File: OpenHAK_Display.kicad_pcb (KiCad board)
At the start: 2 copper layers, 23.4 x 21.7 mm, 13 parts, among them P1 M52-Series_Male_TH_Harwin

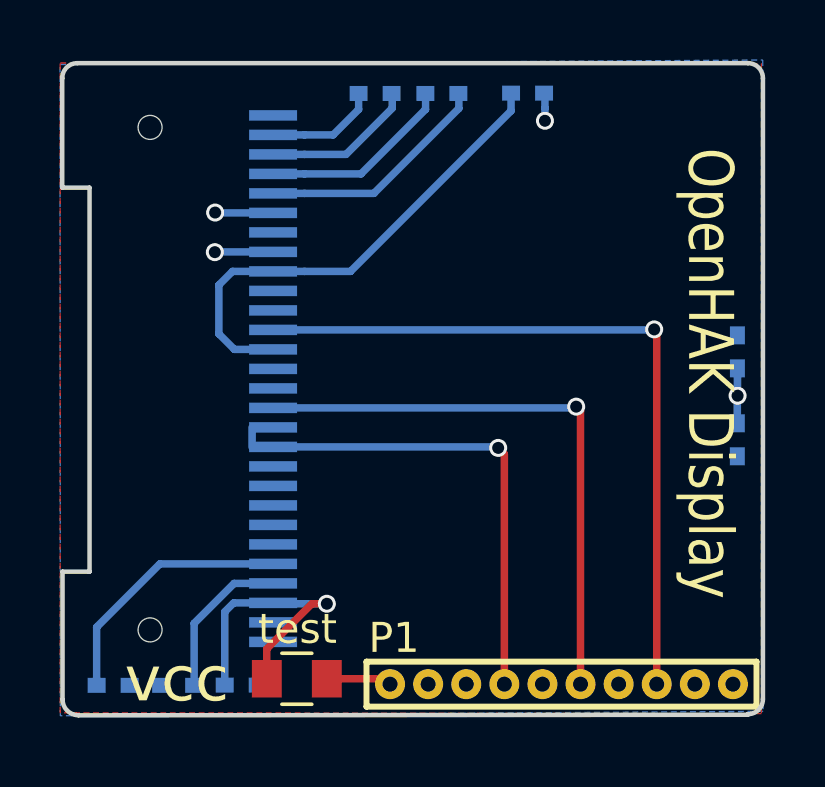
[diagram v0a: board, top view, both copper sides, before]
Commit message: made production files
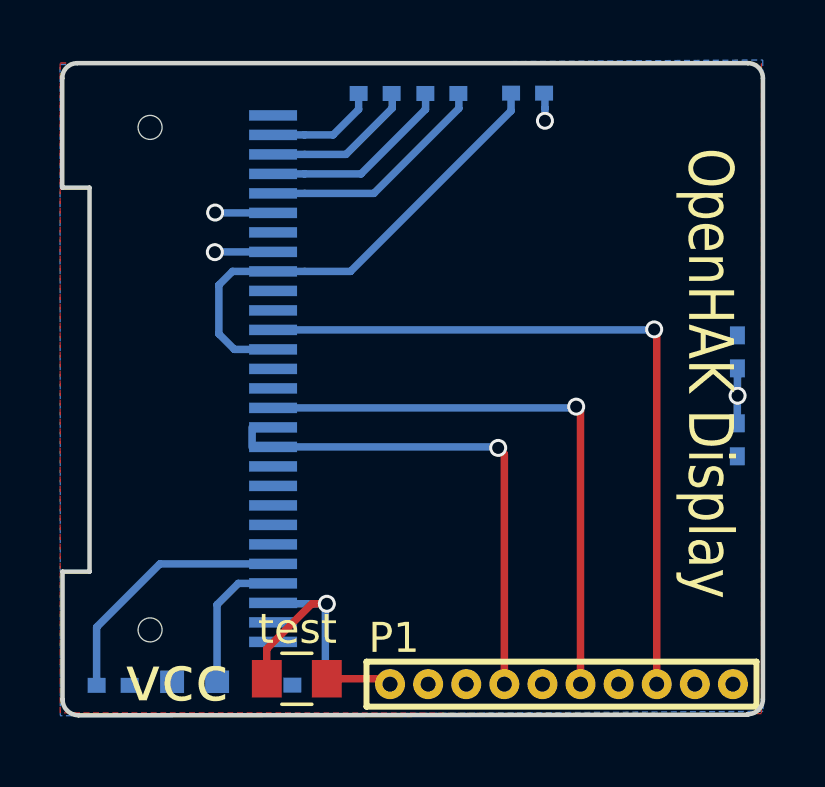
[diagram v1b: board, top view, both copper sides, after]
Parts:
- C3: footprint Capacitors_SMD:C_0402 -> Capacitors_SMD:C_0603
- moved C4 2.25 mm to (125.4, 112.0), turned to 180 degrees
- moved C3 0.58 mm to (121.6, 111.9)
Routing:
- net /VCC: track 9.60 -> 8.16 mm
- net Net-(C3-Pad2): track 5.67 -> 5.15 mm
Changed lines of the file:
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@@
     (thickness 1.6)
     (drawings 30)
-    (tracks 77)
+    (tracks 76)
     (zones 0)
     (modules 13)
@@
     (34 B.Paste user)
     (35 F.Paste user)
-    (36 B.SilkS user)
-    (37 F.SilkS user)
+    (36 B.SilkS user hide)
+    (37 F.SilkS user hide)
     (38 B.Mask user)
     (39 F.Mask user)
@@
     (visible_elements FFFFFF7F)
     (pcbplotparams
-      (layerselection 0x000f4_ffffffff)
+      (layerselection 0x010fc_ffffffff)
       (usegerberextensions false)
       (usegerberattributes false)
@@
   )
   (module Capacitors_SMD:C_0402 (layer B.Cu)
-    (at 121.031338 111.980542)
+    (at 125.405 111.970542 180)
     (descr "Capacitor SMD 0402, reflow soldering, AVX (see smccp.pdf)")
     (tags "capacitor 0402")
     (attr smd)
-    (fp_text reference C3 (at 0.4 -2.05 90) (layer B.SilkS)
-      (effects (font (size 1 1) (thickness 0.15)) (justify mirror))
-    )
-    (fp_text value "4.7uF 16V" (at 0 -1.27) (layer B.Fab)
-      (effects (font (size 1 1) (thickness 0.15)) (justify mirror))
-    )
-    (fp_line (start 1 -0.4) (end -1 -0.4) (layer B.CrtYd) (width 0.05))
-    (fp_line (start 1 -0.4) (end 1 0.4) (layer B.CrtYd) (width 0.05))
-    (fp_line (start -1 0.4) (end -1 -0.4) (layer B.CrtYd) (width 0.05))
-    (fp_line (start -1 0.4) (end 1 0.4) (layer B.CrtYd) (width 0.05))
-    (fp_line (start -0.25 -0.47) (end 0.25 -0.47) (layer B.SilkS) (width 0.12))
-    (fp_line (start 0.25 0.47) (end -0.25 0.47) (layer B.SilkS) (width 0.12))
-    (fp_line (start -0.5 0.25) (end 0.5 0.25) (layer B.Fab) (width 0.1))
-    (fp_line (start 0.5 0.25) (end 0.5 -0.25) (layer B.Fab) (width 0.1))
-    (fp_line (start 0.5 -0.25) (end -0.5 -0.25) (layer B.Fab) (width 0.1))
-    (fp_line (start -0.5 -0.25) (end -0.5 0.25) (layer B.Fab) (width 0.1))
-    (fp_text user %R (at 0 1.27) (layer B.Fab)
-      (effects (font (size 1 1) (thickness 0.15)) (justify mirror))
-    )
-    (pad 2 smd rect (at 0.55 0) (size 0.6 0.5) (layers B.Cu B.Paste B.Mask)
-      (net 5 "Net-(C3-Pad2)"))
-    (pad 1 smd rect (at -0.55 0) (size 0.6 0.5) (layers B.Cu B.Paste B.Mask)
-      (net 6 GND))
-    (model Capacitors_SMD.3dshapes/C_0402.wrl
-      (at (xyz 0 0 0))
-      (scale (xyz 1 1 1))
-      (rotate (xyz 0 0 0))
-    )
-  )
-  (module Capacitors_SMD:C_0402 (layer B.Cu)
-    (at 123.151338 111.970542)
-    (descr "Capacitor SMD 0402, reflow soldering, AVX (see smccp.pdf)")
-    (tags "capacitor 0402")
-    (attr smd)
-    (fp_text reference C4 (at -0.46 -2 90) (layer B.SilkS)
-      (effects (font (size 1 1) (thickness 0.15)) (justify mirror))
-    )
-    (fp_text value 2.2uF (at 0 -1.27) (layer B.Fab)
-      (effects (font (size 1 1) (thickness 0.15)) (justify mirror))
-    )
-    (fp_text user %R (at 0 1.27) (layer B.Fab)
+    (fp_text reference C4 (at -0.46 -2 270) (layer B.SilkS)
+      (effects (font (size 1 1) (thickness 0.15)) (justify mirror))
+    )
+    (fp_text value 2.2uF (at 0 -1.27 180) (layer B.Fab)
+      (effects (font (size 1 1) (thickness 0.15)) (justify mirror))
+    )
+    (fp_text user %R (at 0 1.27 180) (layer B.Fab)
       (effects (font (size 1 1) (thickness 0.15)) (justify mirror))
     )
@@
     (fp_line (start 1 -0.4) (end 1 0.4) (layer B.CrtYd) (width 0.05))
     (fp_line (start 1 -0.4) (end -1 -0.4) (layer B.CrtYd) (width 0.05))
-    (pad 1 smd rect (at -0.55 0) (size 0.6 0.5) (layers B.Cu B.Paste B.Mask)
+    (pad 1 smd rect (at -0.55 0 180) (size 0.6 0.5) (layers B.Cu B.Paste B.Mask)
       (net 26 /VCC))
-    (pad 2 smd rect (at 0.55 0) (size 0.6 0.5) (layers B.Cu B.Paste B.Mask)
+    (pad 2 smd rect (at 0.55 0 180) (size 0.6 0.5) (layers B.Cu B.Paste B.Mask)
       (net 6 GND))
     (model Capacitors_SMD.3dshapes/C_0402.wrl
@@
       (xy 0.376964 2.709982)) (layer B.SilkS) (width 0.01))
   )
+  (module Capacitors_SMD:C_0603 (layer B.Cu)
+    (at 121.595 111.861)
+    (descr "Capacitor SMD 0603, reflow soldering, AVX (see smccp.pdf)")
+    (tags "capacitor 0603")
+    (attr smd)
+    (fp_text reference C3 (at 0 1.5) (layer B.SilkS)
+      (effects (font (size 1 1) (thickness 0.15)) (justify mirror))
+    )
+    (fp_text value "4.7uF 16V" (at 0 -1.5) (layer B.Fab)
+      (effects (font (size 1 1) (thickness 0.15)) (justify mirror))
+    )
+    (fp_text user %R (at 0 0) (layer B.Fab)
+      (effects (font (size 0.3 0.3) (thickness 0.075)) (justify mirror))
+    )
+    (fp_line (start -0.8 -0.4) (end -0.8 0.4) (layer B.Fab) (width 0.1))
+    (fp_line (start 0.8 -0.4) (end -0.8 -0.4) (layer B.Fab) (width 0.1))
+    (fp_line (start 0.8 0.4) (end 0.8 -0.4) (layer B.Fab) (width 0.1))
+    (fp_line (start -0.8 0.4) (end 0.8 0.4) (layer B.Fab) (width 0.1))
+    (fp_line (start -0.35 0.6) (end 0.35 0.6) (layer B.SilkS) (width 0.12))
+    (fp_line (start 0.35 -0.6) (end -0.35 -0.6) (layer B.SilkS) (width 0.12))
+    (fp_line (start -1.4 0.65) (end 1.4 0.65) (layer B.CrtYd) (width 0.05))
+    (fp_line (start -1.4 0.65) (end -1.4 -0.65) (layer B.CrtYd) (width 0.05))
+    (fp_line (start 1.4 -0.65) (end 1.4 0.65) (layer B.CrtYd) (width 0.05))
+    (fp_line (start 1.4 -0.65) (end -1.4 -0.65) (layer B.CrtYd) (width 0.05))
+    (pad 1 smd rect (at -0.75 0) (size 0.8 0.75) (layers B.Cu B.Paste B.Mask)
+      (net 6 GND))
+    (pad 2 smd rect (at 0.75 0) (size 0.8 0.75) (layers B.Cu B.Paste B.Mask)
+      (net 5 "Net-(C3-Pad2)"))
+    (model Capacitors_SMD.3dshapes/C_0603.wrl
+      (at (xyz 0 0 0))
+      (scale (xyz 1 1 1))
+      (rotate (xyz 0 0 0))
+    )
+  )
   (gr_text vcc (at 121.005 111.786) (layer F.SilkS)
     (effects (font (size 1.5 1.5) (thickness 0.3)))
@@
   (segment (start 123.926351 108.581958) (end 123.931952 108.587559) (width 0.254) (layer B.Cu) (net 5))
   (segment (start 123.512752 108.581959) (end 123.926351 108.581958) (width 0.254) (layer B.Cu) (net 5))
-  (segment (start 122.913511 108.581959) (end 124.212752 108.581959) (width 0.25) (layer B.Cu) (net 5))
-  (segment (start 121.581338 109.914132) (end 122.913511 108.581959) (width 0.25) (layer B.Cu) (net 5))
-  (segment (start 121.581338 111.980542) (end 121.581338 109.914132) (width 0.25) (layer B.Cu) (net 5))
+  (segment (start 122.345 111.861) (end 122.345 109.291) (width 0.25) (layer B.Cu) (net 5))
+  (segment (start 123.054041 108.581959) (end 124.212752 108.581959) (width 0.25) (layer B.Cu) (net 5))
+  (segment (start 122.345 109.291) (end 123.054041 108.581959) (width 0.25) (layer B.Cu) (net 5))
   (segment (start 127.931796 111.761) (end 128.111338 111.940542) (width 0.25) (layer F.Cu) (net 6))
   (segment (start 126.005 111.761) (end 127.931796 111.761) (width 0.25) (layer F.Cu) (net 6))
@@
   (segment (start 120.439921 107.931959) (end 124.212752 107.931958) (width 0.25) (layer B.Cu) (net 20))
   (segment (start 118.331338 110.040542) (end 120.439921 107.931959) (width 0.25) (layer B.Cu) (net 20))
-  (segment (start 122.601338 111.970542) (end 122.601338 109.530542) (width 0.25) (layer B.Cu) (net 26))
-  (segment (start 122.899921 109.231959) (end 124.212752 109.231959) (width 0.25) (layer B.Cu) (net 26))
-  (segment (start 122.601338 109.530542) (end 122.899921 109.231959) (width 0.25) (layer B.Cu) (net 26))
   (via (at 126.005 109.261) (size 0.6) (drill 0.4) (layers F.Cu B.Cu) (net 26))
   (segment (start 124.241793 109.261) (end 124.212752 109.231959) (width 0.25) (layer B.Cu) (net 26))
@@
   (segment (start 124.005 110.761) (end 125.505 109.261) (width 0.25) (layer F.Cu) (net 26))
   (segment (start 124.005 111.761) (end 124.005 110.761) (width 0.25) (layer F.Cu) (net 26))
+  (segment (start 125.955 109.311) (end 126.005 109.261) (width 0.25) (layer B.Cu) (net 26))
+  (segment (start 125.955 111.970542) (end 125.955 109.311) (width 0.25) (layer B.Cu) (net 26))
   (zone (net 7) (net_name +3V3) (layer F.Cu) (hatch edge 0.508)
     (connect_pads (clearance 0.2))
